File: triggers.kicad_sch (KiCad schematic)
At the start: 19 parts, among them U10 SN74LVC2G17DB, U13 SRV05-4, U9 SN74LVC2G17DB

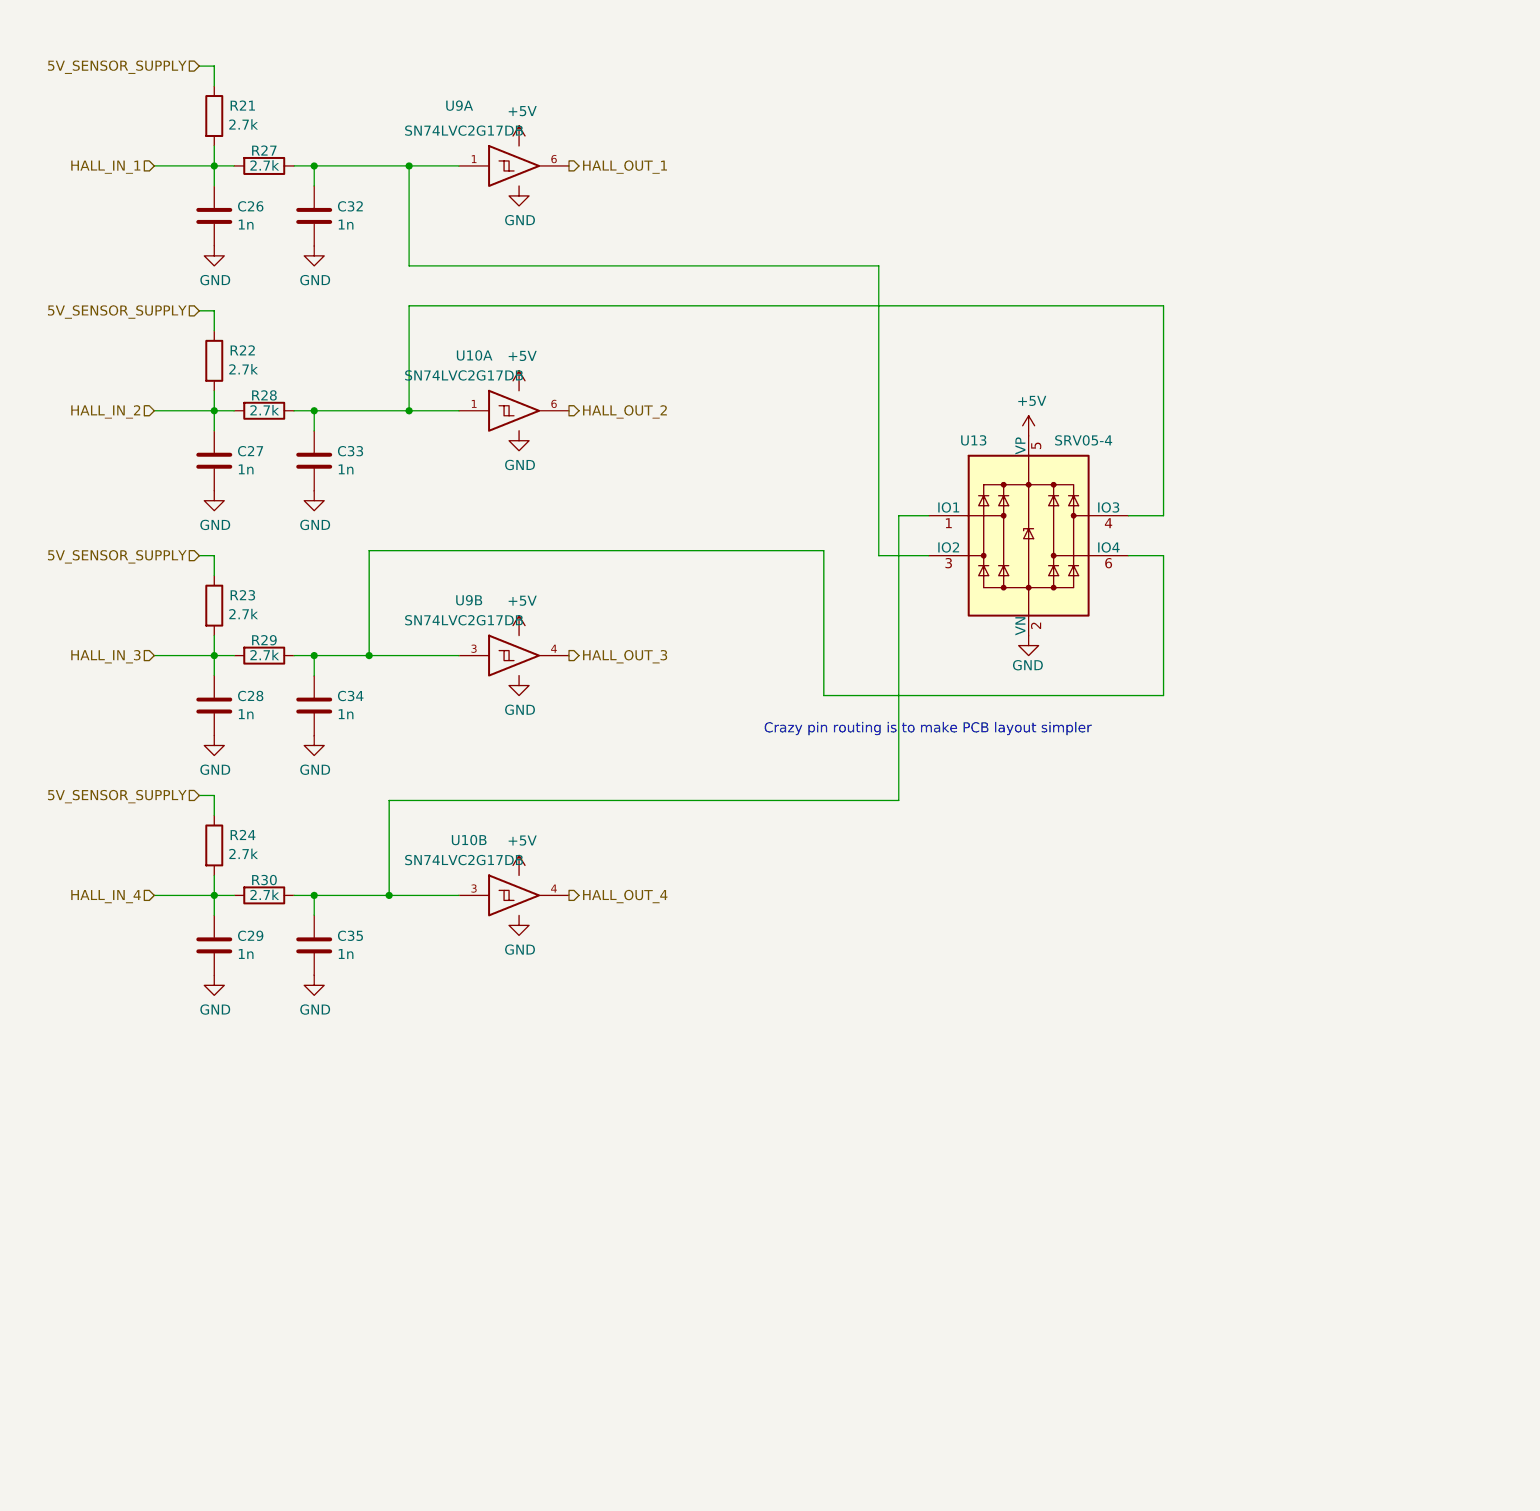
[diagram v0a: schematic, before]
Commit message: Several optimizations
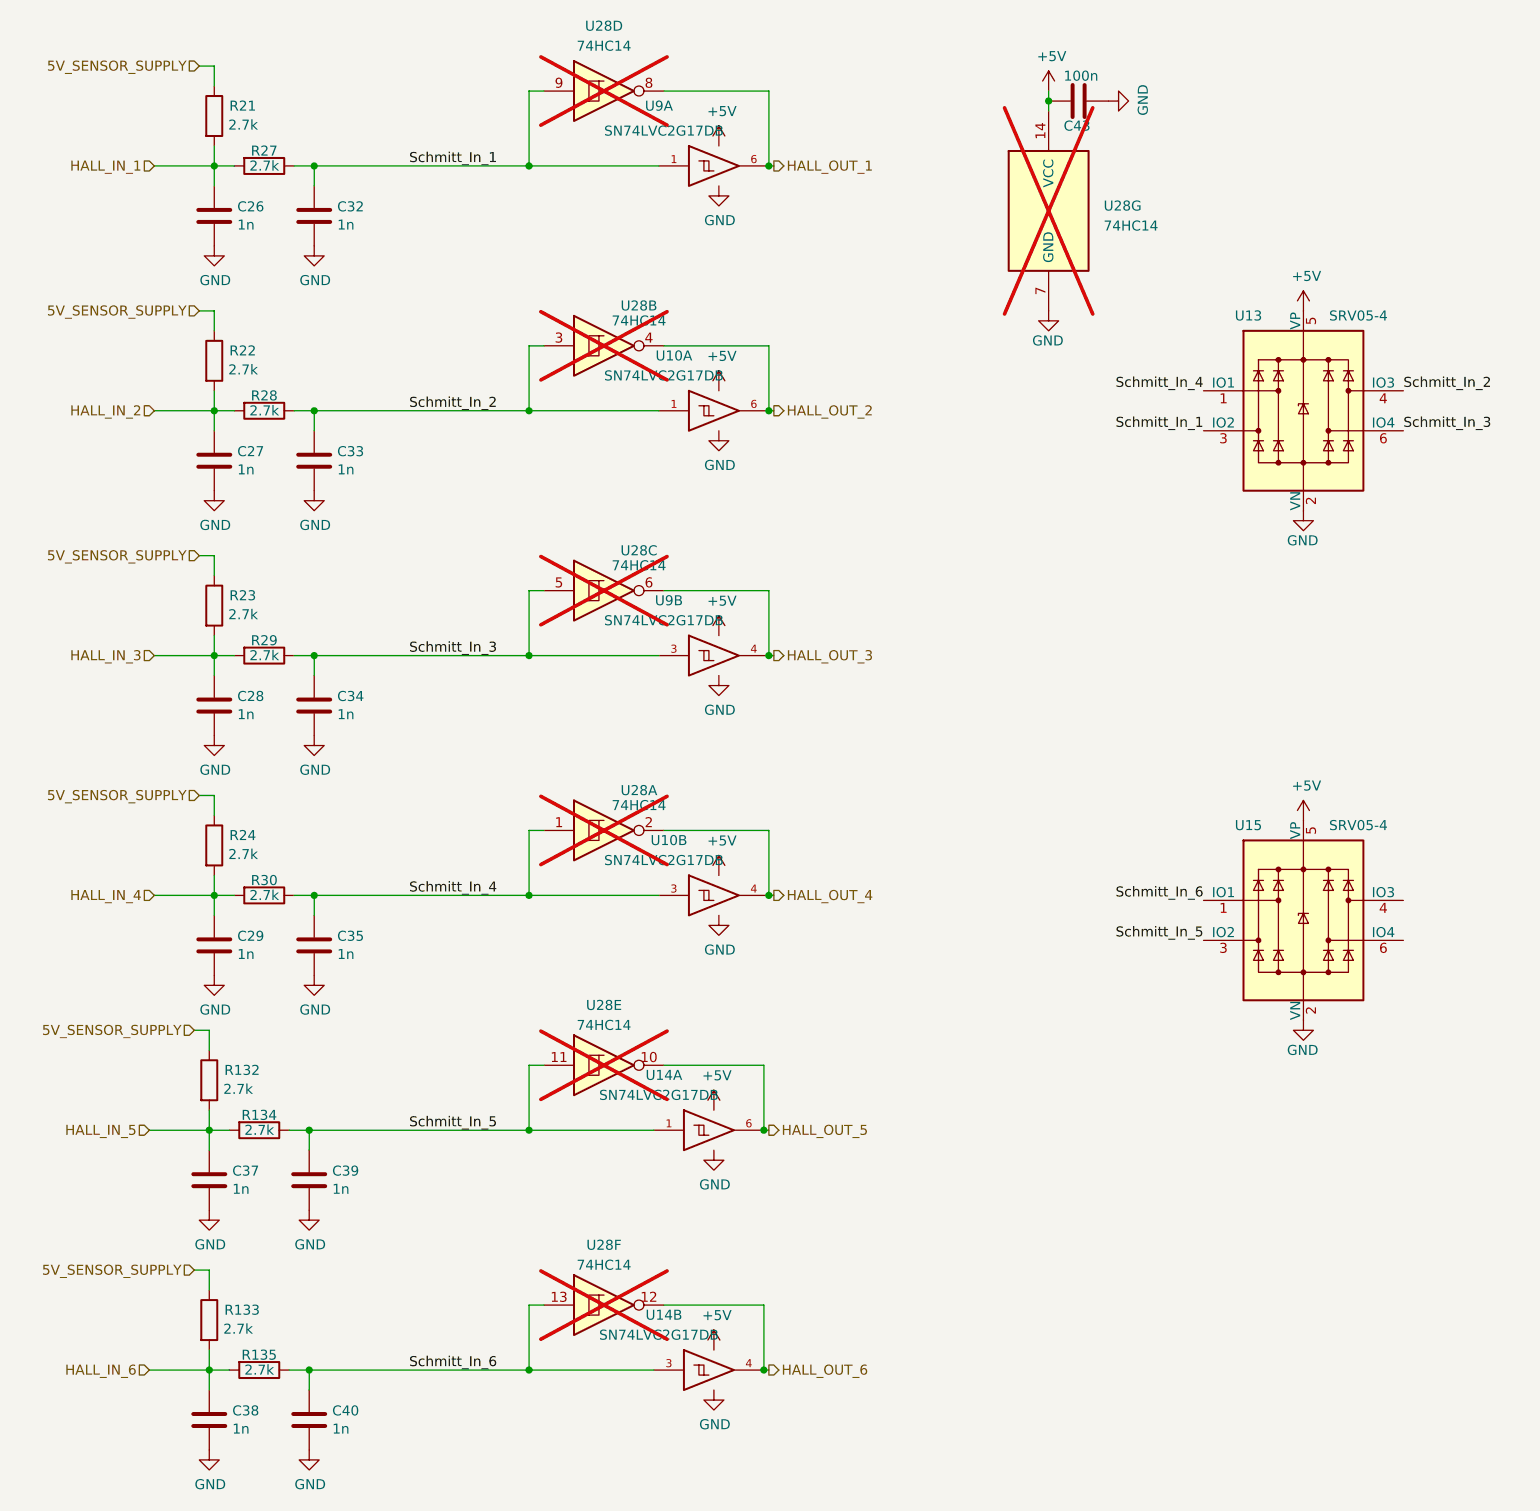
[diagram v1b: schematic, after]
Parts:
- added C37, C38, C39, C40: 1n, Capacitor_SMD:C_0603_1608Metric, symbol Device:C
- added C43: 100n, Capacitor_SMD:C_0603_1608Metric, symbol Device:C
- added R132, R133, R134, R135: 2.7k, Resistor_SMD:R_0603_1608Metric, symbol Device:R
- added U14: SN74LVC2G17DB, Package_TO_SOT_SMD:SOT-23-6, symbol 74xGxx:74LVC2G17
- added U15: SRV05-4, Package_TO_SOT_SMD:SOT-23-6, symbol Power_Protection:SRV05-4
- added U28: 74HC14, SOIC-14_3.9x8.7mm_P1.27mm, symbol 74xx:74HC14
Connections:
- net +5V: now also C43.2, U14.5 (VCC), U14.5 (VCC), U15.5 (VP), U28.14 (VCC)
- net 5V_SENSOR_SUPPLY: now also R132.1, R133.1
- net GND: now also C37.2, C38.2, C39.2, C40.2, C43.1, U14.2 (GND), U14.2 (GND), U15.2 (VN), U28.7 (GND)
- net HALL_OUT_1: now also U28.8
- net HALL_OUT_2: now also U28.4
- net HALL_OUT_3: now also U28.6
- net HALL_OUT_4: now also U28.2
- net Schmitt_In_1: now reaches C32.1, R27.1, U13.3 (IO2), U9.1
- net Schmitt_In_1: now also U28.9
- net Schmitt_In_2: now reaches C33.1, R28.1, U10.1, U13.4 (IO3)
- net Schmitt_In_2: now also U28.3
- net Schmitt_In_3: now reaches C34.1, R29.1, U13.6 (IO4), U9.3
- net Schmitt_In_3: now also U28.5
- net Schmitt_In_4: now reaches C35.1, R30.1, U10.3, U13.1 (IO1)
- net Schmitt_In_4: now also U28.1
- new net HALL_IN_5: C37.1, R132.2, R134.2
- new net HALL_IN_6: C38.1, R133.2, R135.2
- new net HALL_OUT_5: U14.6, U28.10
- new net HALL_OUT_6: U14.4, U28.12
- new net Schmitt_In_5: C39.1, R134.1, U14.1, U15.3 (IO2), U28.11
- new net Schmitt_In_6: C40.1, R135.1, U14.3, U15.1 (IO1), U28.13
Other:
- note removed: "Crazy pin routing is to make PCB layout simpler"
- moved on the sheet: U10A, U10B, U13, U9A, U9B
